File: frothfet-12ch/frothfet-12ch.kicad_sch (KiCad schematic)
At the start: 8 parts

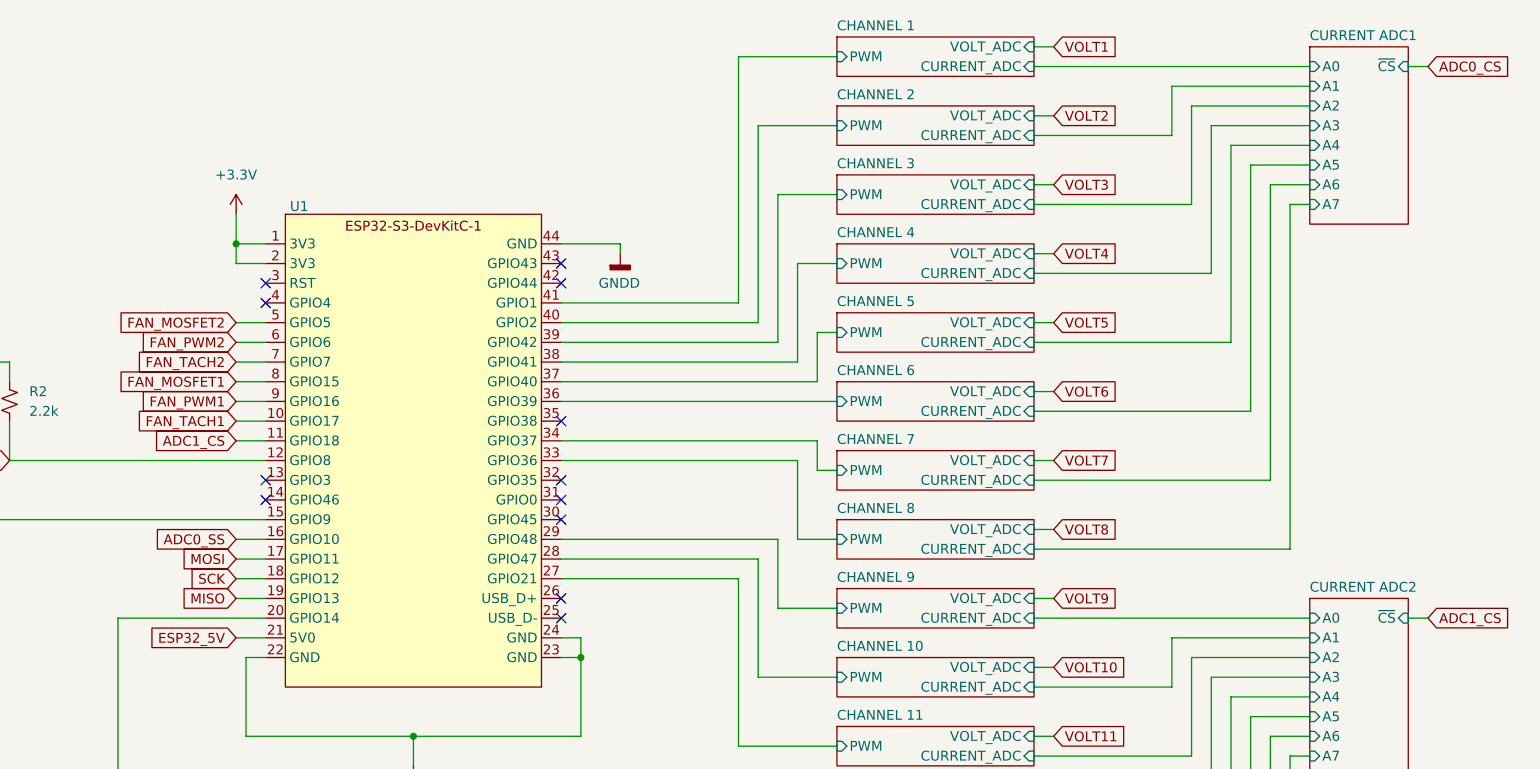
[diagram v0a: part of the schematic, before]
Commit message: schematic looking clean.
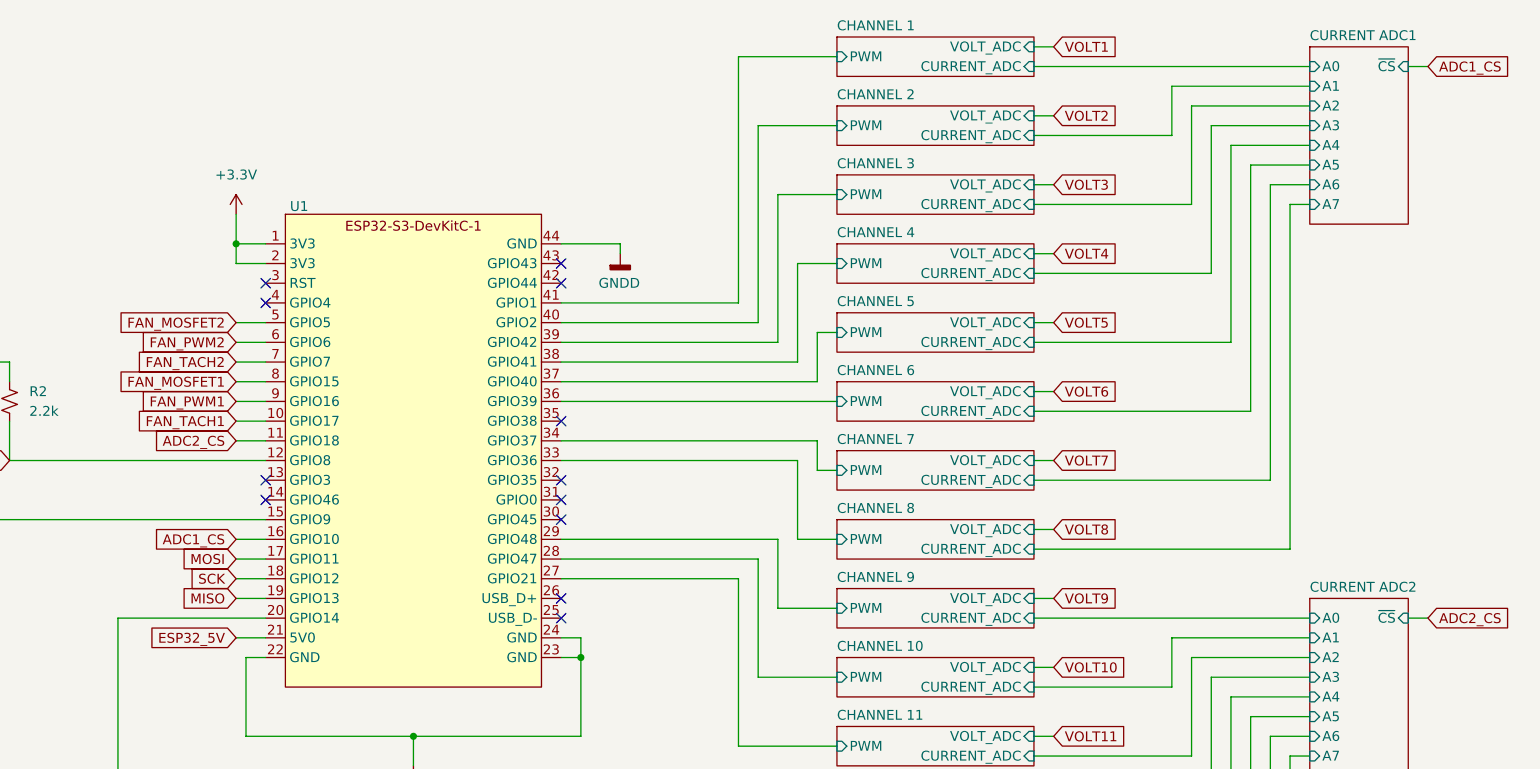
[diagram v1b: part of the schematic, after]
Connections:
- net ADC0_SS is gone; now on net ADC1_CS: U1.16 (GPIO10)
- net ADC1_CS: no longer U1.11 (GPIO18)
- new net ADC2_CS: U1.11 (GPIO18)
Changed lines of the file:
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@@
 		)
 	)
-	(global_label "ADC0_CS"
+	(global_label "ADC1_CS"
 		(shape input)
 		(at 270.51 36.83 0)
@@
 		)
 	)
-	(global_label "ADC0_SS"
+	(global_label "ADC1_CS"
 		(shape input)
 		(at 116.84 97.79 180)
@@
 		)
 		(property "Intersheetrefs" "${INTERSHEET_REFS}"
-			(at 105.6301 97.79 0)
+			(at 105.5696 97.79 0)
 			(effects
 				(font
@@
 		)
 	)
-	(global_label "ADC1_CS"
+	(global_label "ADC2_CS"
 		(shape input)
 		(at 270.51 107.95 0)
@@
 		)
 	)
-	(global_label "ADC1_CS"
+	(global_label "ADC2_CS"
 		(shape input)
 		(at 116.84 85.09 180)
